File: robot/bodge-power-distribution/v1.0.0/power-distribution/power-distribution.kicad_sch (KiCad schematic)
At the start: 5 parts, among them J1 Conn_01x02, SW1 SW_SPST

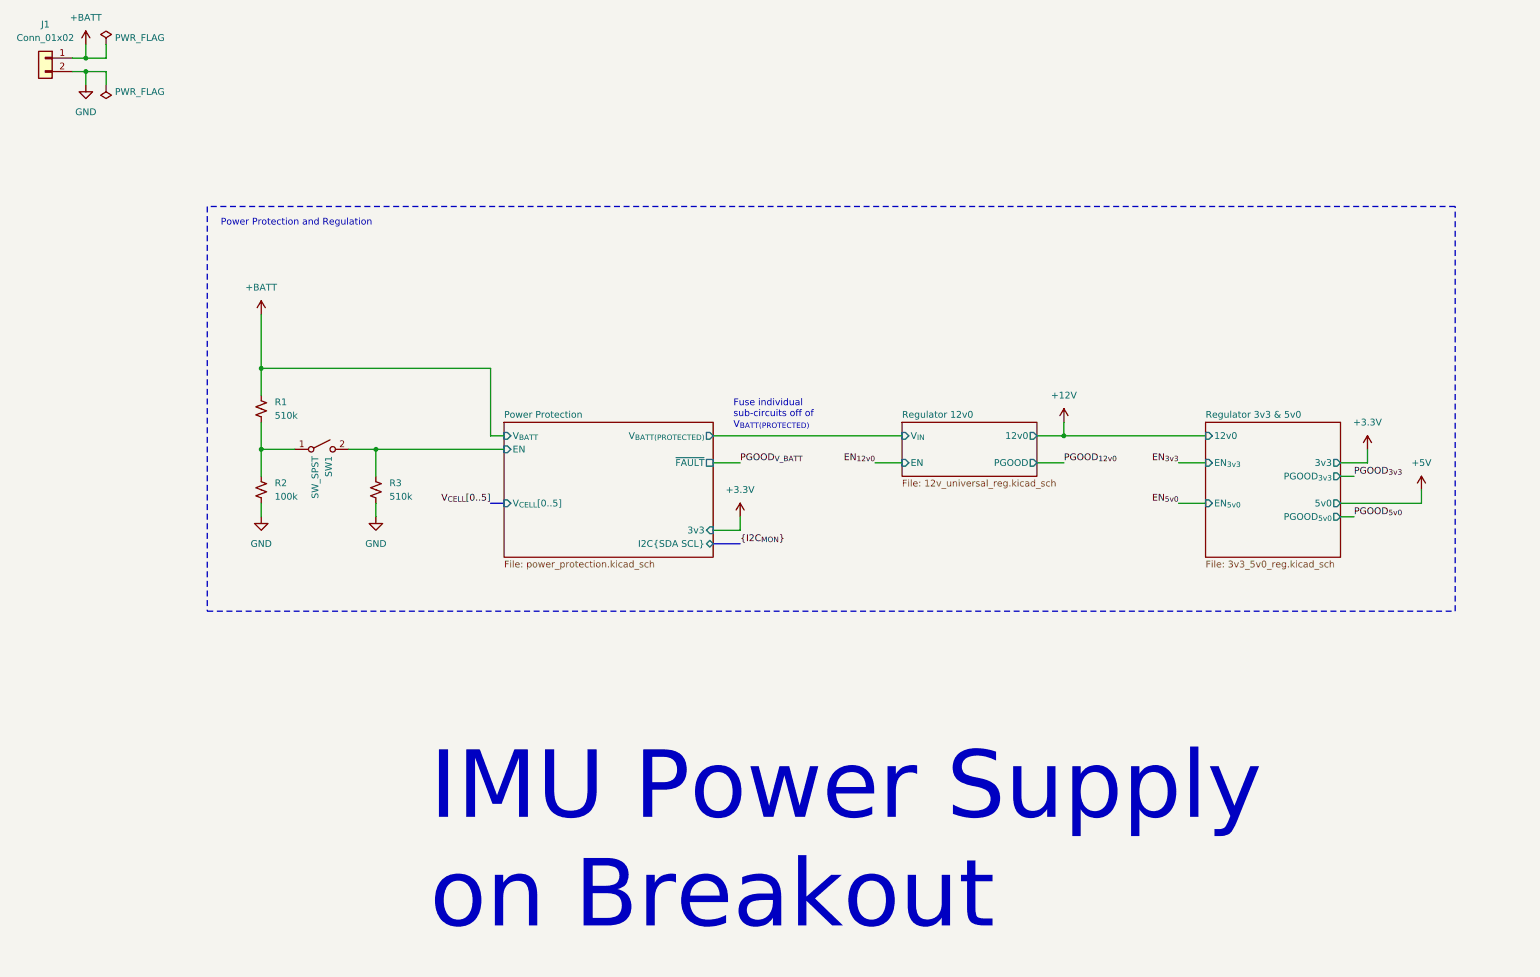
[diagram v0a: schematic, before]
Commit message: Sync
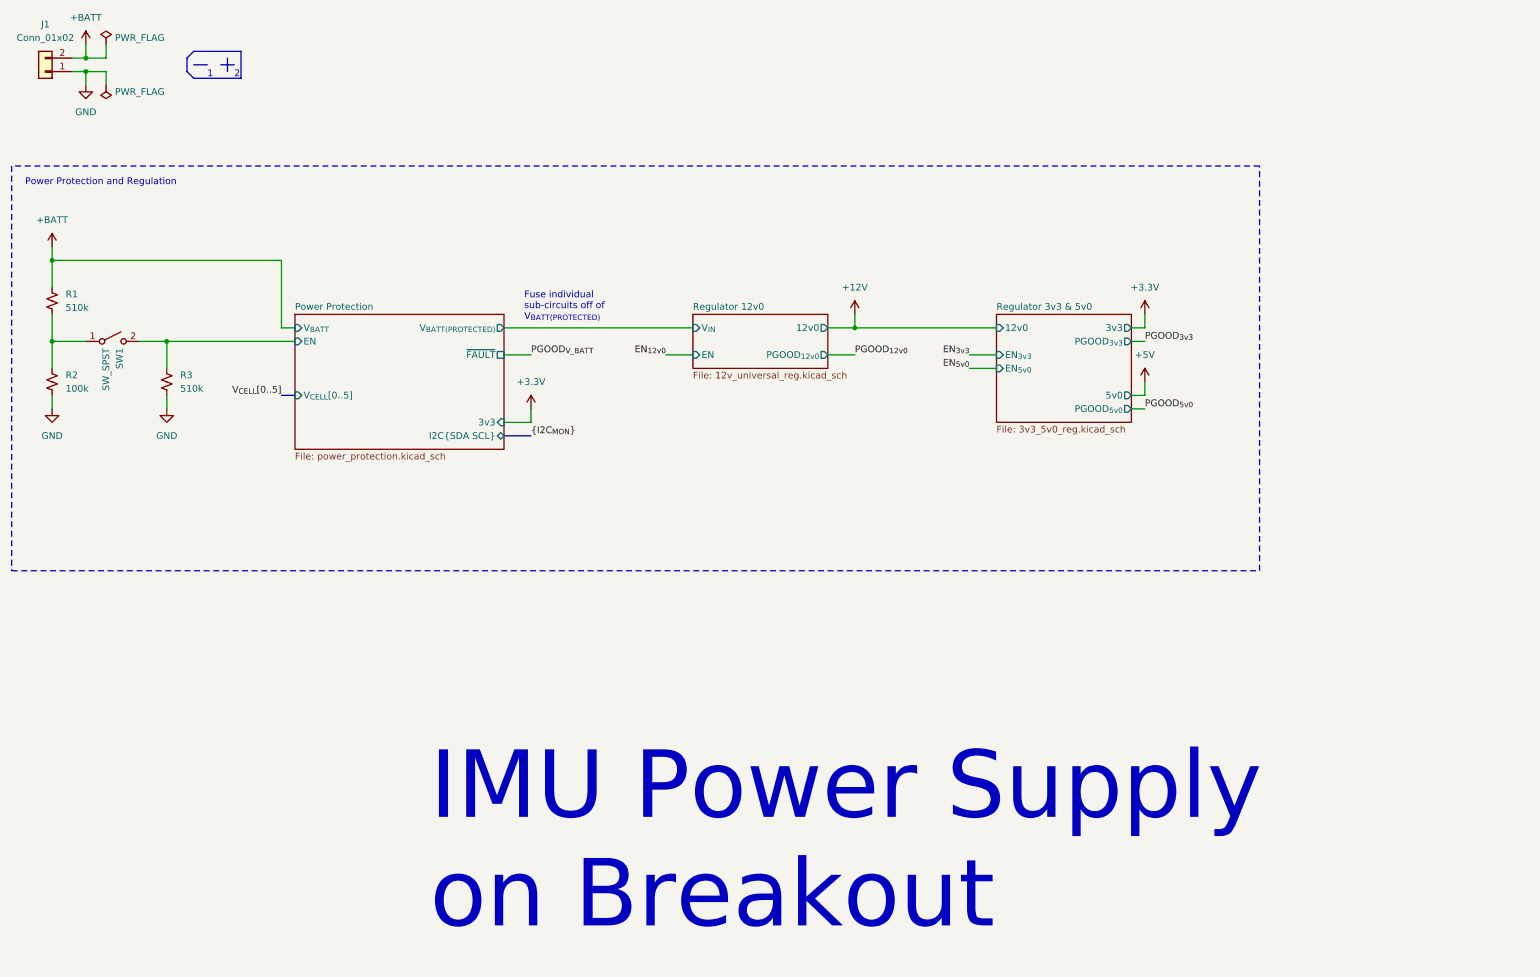
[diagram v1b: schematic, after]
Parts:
- J1: footprint (none) -> Connector_AMASS:AMASS_XT60-M_1x02_P7.20mm_Vertical
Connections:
- net +BATT: now also J1.2 (Pin_2); no longer J1.1 (Pin_1)
- net GND: now also J1.1 (Pin_1); no longer J1.2 (Pin_2)
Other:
- sheet Regulator 12v0 ports: added PGOOD_{12v0}; removed PGOOD
- note added: "1"
- note added: "2"
- moved on the sheet: J1, R1, R2, R3, SW1
